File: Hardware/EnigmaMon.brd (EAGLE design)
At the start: 100 x 80 mm, 57 parts, among them IC1 4051N, IC2 TLC5940, IC3 MEGA8-P, T1 BC548, T2 BC548, T3 BC548, T4 BC548, T5 BC548, T6 BC548, T8 BC548, T9 BC548

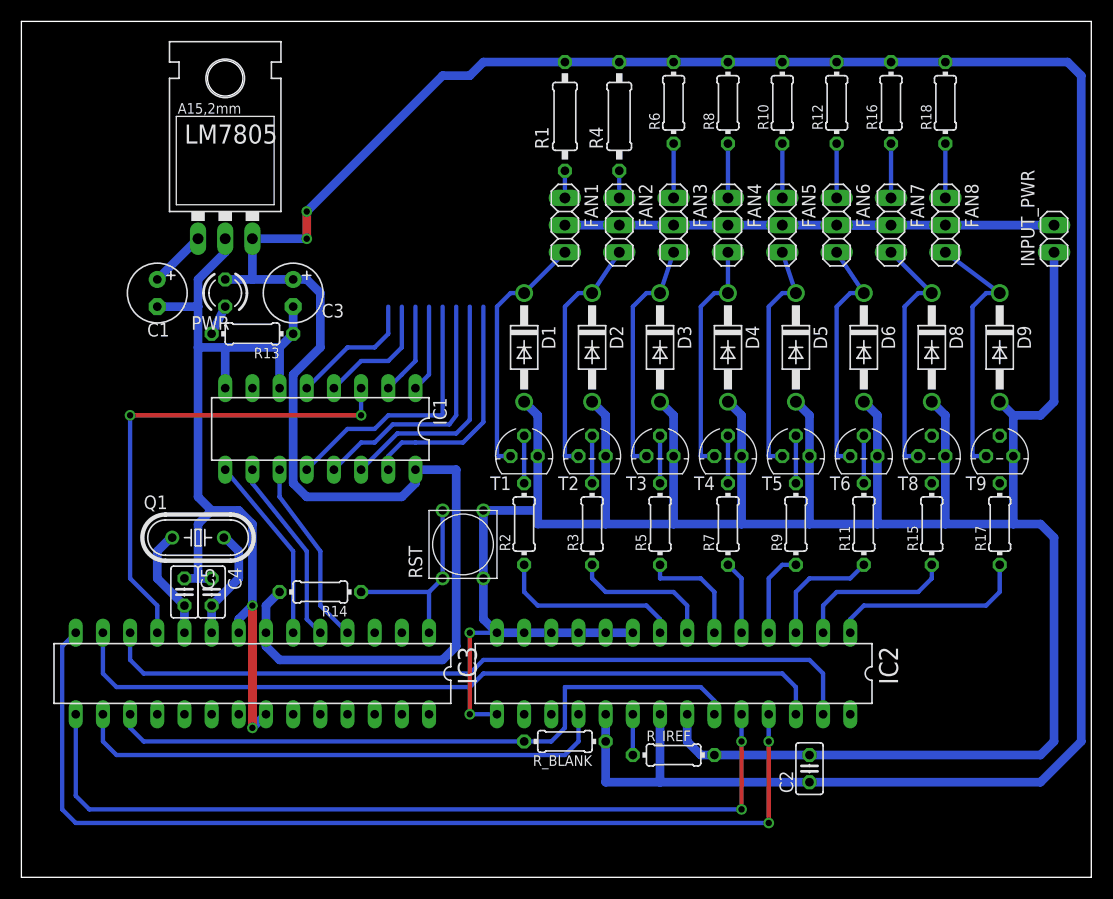
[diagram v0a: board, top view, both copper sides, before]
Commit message: Testing
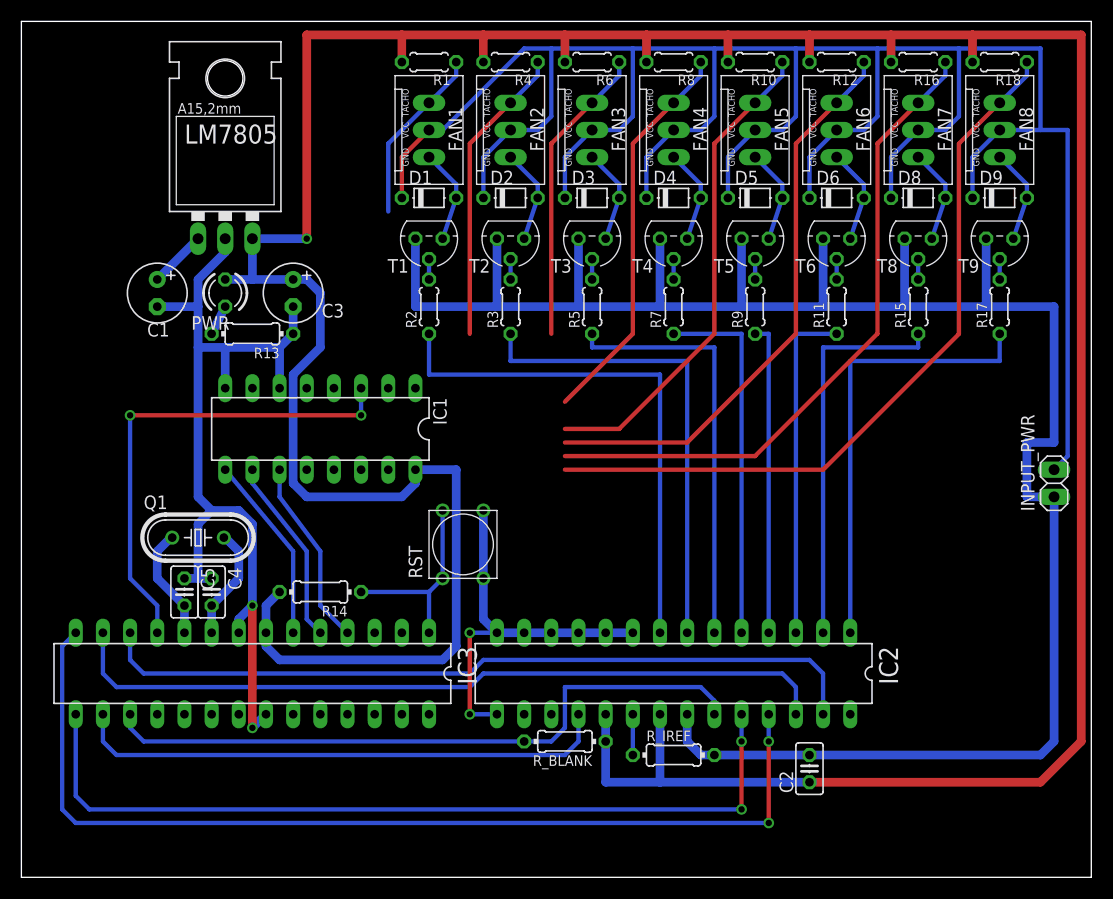
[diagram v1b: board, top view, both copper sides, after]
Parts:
- D1, D2, D3, D4, D5, D6, D8, D9: value 1N4004 -> (none); device diode:DO41-10 -> diode:D-5
- FAN1, FAN2, FAN3, FAN4, FAN5, FAN6, FAN7, FAN8: value (none) -> FAN; device pinhead:1X03 -> EnigmaMon:FAN_HEADER
- R1, R4: device rcl:0207/10 -> rcl:0204/5
- R10, R11, R12, R15, R16, R17, R18, R2, R3, R5, R6, R7, R8, R9: device rcl:0204/7 -> rcl:0204/5
- moved INPUT_PWR 22.9 mm to (96.5, 36.8)
- moved R2 22.2 mm to (38.1, 53.3)
- moved T1 22.2 mm to (38.1, 59.7), turned to 180 degrees
- moved R3 21.7 mm to (45.7, 53.3)
- moved T2 21.7 mm to (45.7, 59.7), turned to 180 degrees
- moved R5 21.3 mm to (53.3, 53.3)
- moved T3 21.3 mm to (53.3, 59.7), turned to 180 degrees
- moved R7 20.9 mm to (61.0, 53.3)
- moved T4 20.9 mm to (61.0, 59.7), turned to 180 degrees
- moved R9 20.7 mm to (68.6, 53.3)
- moved T5 20.7 mm to (68.6, 59.7), turned to 180 degrees
- moved R11 20.5 mm to (76.2, 53.3)
- moved T6 20.5 mm to (76.2, 59.7), turned to 180 degrees
- moved R15 20.4 mm to (83.8, 53.3)
- moved T8 20.4 mm to (83.8, 59.7), turned to 180 degrees
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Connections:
- removed net FAN1_GND: D1.C, FAN1.3, T1.3
- removed net FAN2_GND: D2.C, FAN2.3, T2.3
- removed net FAN3_GND: D3.C, FAN3.3, T3.3
- removed net FAN4_GND: D4.C, FAN4.3, T4.3
- removed net FAN5_GND: D5.C, FAN5.3, T5.3
- removed net FAN6_GND: D6.C, FAN6.3, T6.3
- removed net FAN7_GND: D8.C, FAN7.3, T8.3
- removed net FAN8_GND: D9.C, FAN8.3, T9.3
- new net N$13: D2.A, FAN2.GND, T2.3
- new net N$14: D3.A, FAN3.GND, T3.3
- new net N$15: D4.A, FAN4.GND, T4.3
- new net N$16: D1.A, FAN1.GND, T1.3
- new net N$17: D9.A, FAN8.GND, T9.3
- new net N$19: D8.A, FAN7.GND, T8.3
- new net N$20: D6.A, FAN6.GND, T6.3
- new net N$21: D5.A, FAN5.GND, T5.3
- net +12V: now also D1.C, D2.C, D3.C, D4.C, D5.C, D6.C, D8.C, D9.C, FAN1.VCC, FAN2.VCC, FAN3.VCC, FAN4.VCC, FAN5.VCC, FAN6.VCC, FAN7.VCC, FAN8.VCC; no longer FAN1.2, FAN2.2, FAN3.2, FAN4.2, FAN5.2, FAN6.2, FAN7.2, FAN8.2
- net FAN1_TACHO: now also FAN1.TACHO; no longer FAN1.1
- net FAN2_TACHO: now also FAN2.TACHO; no longer FAN2.1
- net FAN3_TACHO: now also FAN3.TACHO; no longer FAN3.1
- net FAN4_TACHO: now also FAN4.TACHO; no longer FAN4.1
- net FAN5_TACHO: now also FAN5.TACHO; no longer FAN5.1
- net FAN6_TACHO: now also FAN6.TACHO; no longer FAN6.1
- net FAN7_TACHO: now also FAN7.TACHO; no longer FAN7.1
- net FAN8_TACHO: now also FAN8.TACHO; no longer FAN8.1
- net GND: no longer D1.A, D2.A, D3.A, D4.A, D5.A, D6.A, D8.A, D9.A
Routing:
- net +12V: track 56.2 -> 235.3 mm
- net FAN8_TACHO: track 13.2 -> 70.1 mm
- net FAN6_TACHO: track 13.8 -> 53.8 mm
- net FAN7_TACHO: track 27.4 -> 62.0 mm
- net VCC: track 297.8 -> 332.2 mm, vias 2 -> 1
- net FAN1_PWM: track 17.6 -> 49.5 mm
- net FAN2_PWM: track 13.8 -> 44.4 mm
- net GND: track 350.1 -> 319.5 mm
- net FAN3_PWM: track 10.7 -> 39.4 mm
- net FAN4_PWM: track 6.88 -> 34.3 mm
- net FAN8_GND: track 24.7 -> 0.00 mm
- net FAN7_GND: track 23.7 -> 0.00 mm
- net FAN1_GND: track 23.7 -> 0.00 mm
- net FAN8_PWM: track 18.8 -> 41.9 mm
- net FAN2_GND: track 22.9 -> 0.00 mm
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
